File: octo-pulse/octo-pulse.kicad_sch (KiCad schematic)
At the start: 8 parts, among them SW1 SW_Push, SW2 SW_Push, SW3 SW_Push, SW4 SW_Push, SW5 SW_Push, SW6 SW_Push

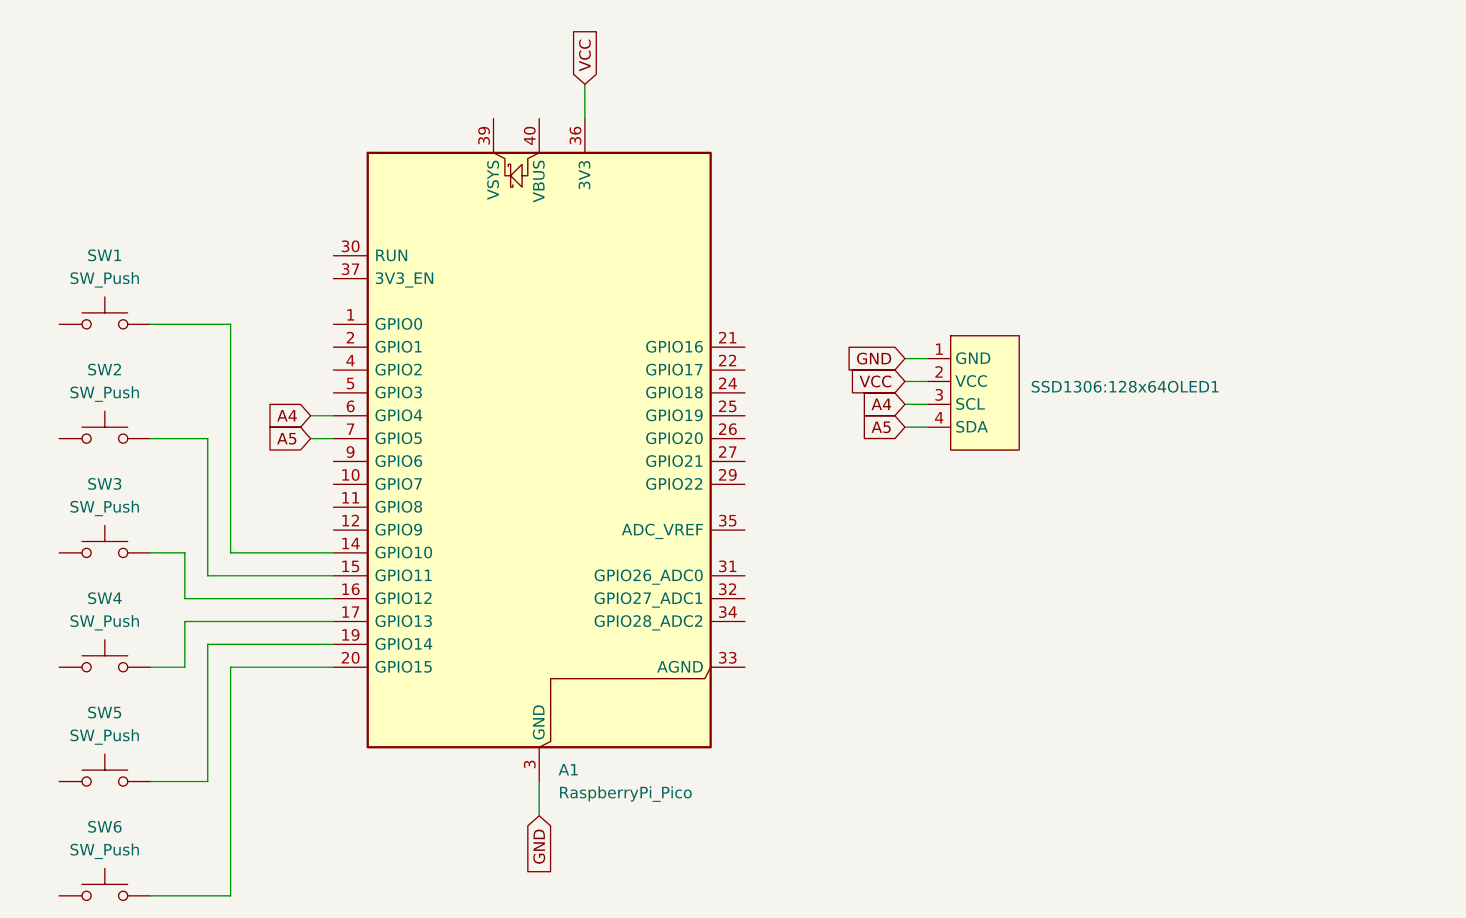
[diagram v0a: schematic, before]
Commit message: Fully wired PCB in KiCad
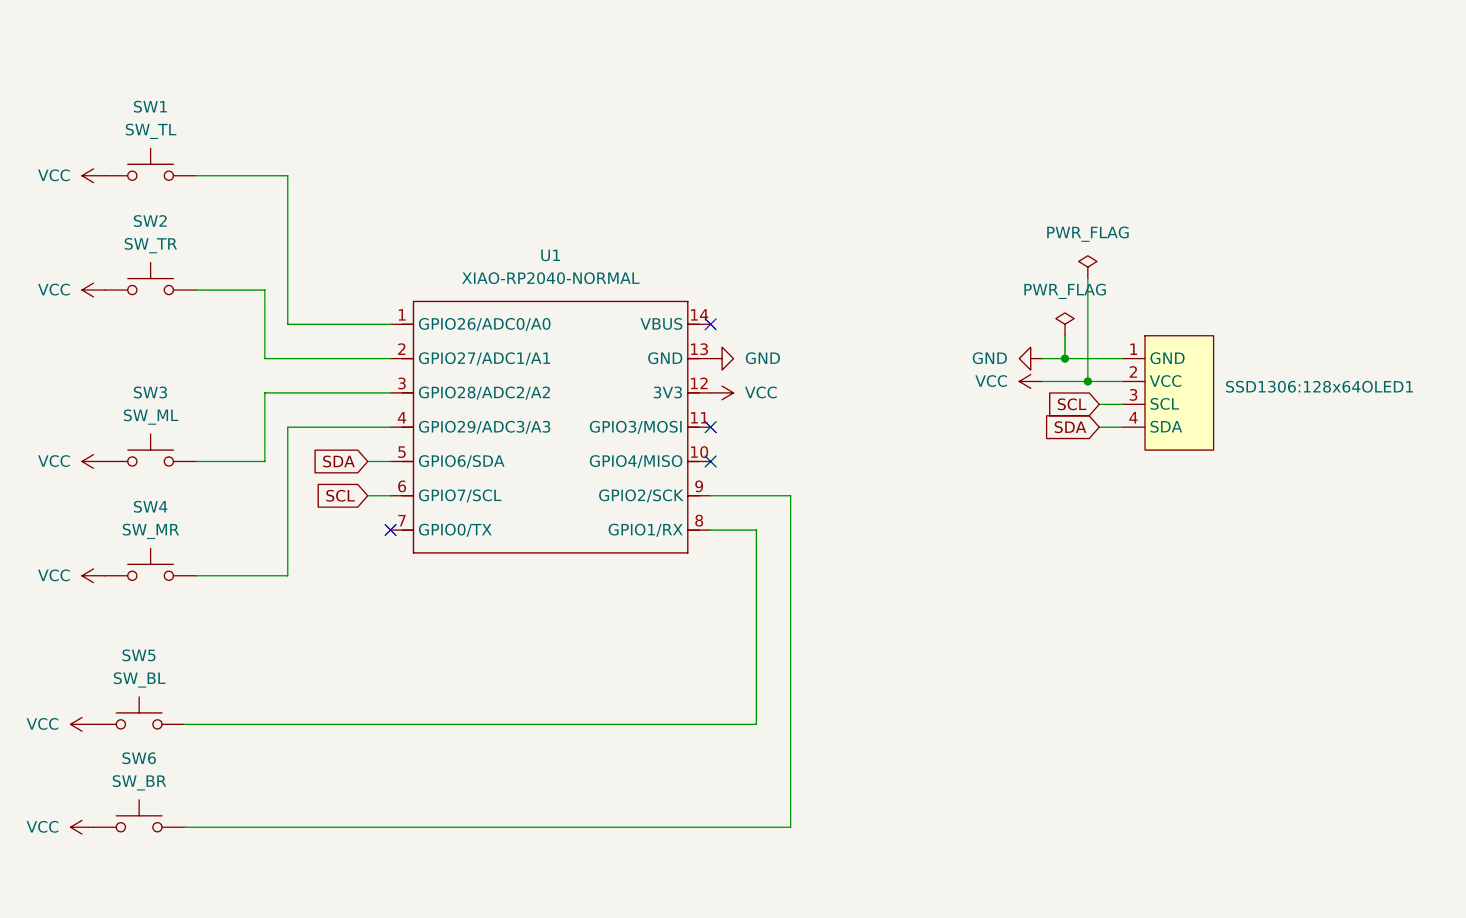
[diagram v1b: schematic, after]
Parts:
- removed A1: RaspberryPi_Pico, Module:RaspberryPi_Pico_Common_Unspecified, symbol MCU_Module:RaspberryPi_Pico
- added U1: XIAO-RP2040-NORMAL, Seeed Studio XIAO Series Library:XIAO-RP2040-DIP, symbol Seeed_Studio_XIAO_Series:XIAO-RP2040-NORMAL
- SSD1306:128x64OLED1: footprint SSD1306:Adafruit_SSD1306_0.96'' -> SSD1306:Adafruit_SSD1306_1.3''
- SW1: value SW_Push -> SW_TL
- SW2: value SW_Push -> SW_TR
- SW3: value SW_Push -> SW_ML
- SW4: value SW_Push -> SW_MR
- SW5: value SW_Push -> SW_BL
- SW6: value SW_Push -> SW_BR
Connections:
- net GND: now also U1.13 (GND)
- net VCC: now also SW1.1, SW2.1, SW3.1, SW4.1, SW5.1, SW6.1, U1.12 (3V3)
- net at SW4.2: now also U1.4 (GPIO29/ADC3/A3)
- net at SW2.2: now also U1.2 (GPIO27/ADC1/A1)
- net at SW1.2: now also U1.1 (GPIO26/ADC0/A0)
- net at SW3.2: now also U1.3 (GPIO28/ADC2/A2)
- net at SW5.2: now also U1.8 (GPIO1/RX)
- net at SW6.2: now also U1.9 (GPIO2/SCK)
- net A4 renamed SCL
- net SCL: now also U1.6 (GPIO7/SCL)
- net A5 renamed SDA
- net SDA: now also U1.5 (GPIO6/SDA)
- no-connect marks 0 -> 4
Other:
- moved on the sheet: SSD1306:128x64OLED1, SW1, SW2, SW3, SW4, SW5, SW6

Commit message: Finished & decorated PCB, onto programming!
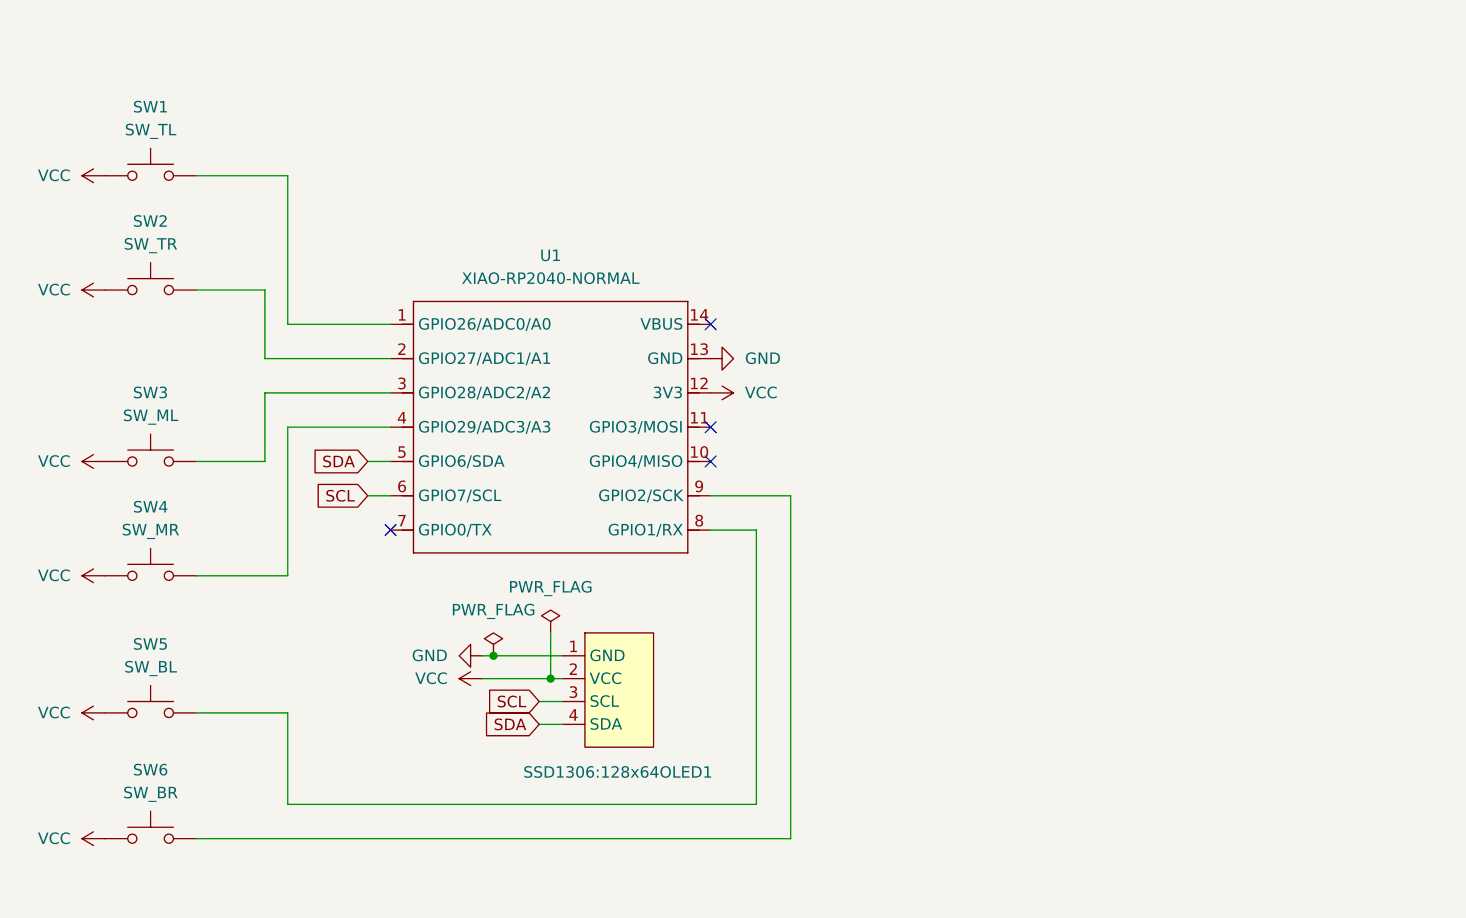
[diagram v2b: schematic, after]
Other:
- moved on the sheet: SSD1306:128x64OLED1, SW5, SW6

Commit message: replaced switches on PCB with new ones: B3U-1000P & B3U-3000P-B
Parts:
- SW1, SW2: footprint EVQ-P7A01P:EVQ_P7_PAN -> B3U-3000P-B:SW_B3U-3000P-B_OMR
- SW3, SW4, SW5, SW6: footprint EVQ-Q2K03W:EVQ-Q2K03W_PAN -> B3U-1000P:B3U-1000P
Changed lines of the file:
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@@
 			)
 		)
-		(property "Footprint" "EVQ-Q2K03W:EVQ-Q2K03W_PAN"
+		(property "Footprint" "B3U-1000P:B3U-1000P"
 			(at 91.44 99.06 0)
 			(effects
@@
 			)
 		)
-		(property "Footprint" "EVQ-P7A01P:EVQ_P7_PAN"
+		(property "Footprint" "B3U-3000P-B:SW_B3U-3000P-B_OMR"
 			(at 91.44 67.31 0)
 			(effects
@@
 			)
 		)
-		(property "Footprint" "EVQ-Q2K03W:EVQ-Q2K03W_PAN"
+		(property "Footprint" "B3U-1000P:B3U-1000P"
 			(at 91.44 114.3 0)
 			(effects
@@
 			)
 		)
-		(property "Footprint" "EVQ-Q2K03W:EVQ-Q2K03W_PAN"
+		(property "Footprint" "B3U-1000P:B3U-1000P"
 			(at 91.44 128.27 0)
 			(effects
@@
 			)
 		)
-		(property "Footprint" "EVQ-Q2K03W:EVQ-Q2K03W_PAN"
+		(property "Footprint" "B3U-1000P:B3U-1000P"
 			(at 91.44 86.36 0)
 			(effects
@@
 			)
 		)
-		(property "Footprint" "EVQ-P7A01P:EVQ_P7_PAN"
+		(property "Footprint" "B3U-3000P-B:SW_B3U-3000P-B_OMR"
 			(at 91.44 54.61 0)
 			(effects
